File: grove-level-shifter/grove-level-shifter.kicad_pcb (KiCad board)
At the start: 2 copper layers, 21.6 x 45.7 mm, 14 parts, among them J1 In 1, J2 In 2, J3 Out 1, J4 Out 2, J5 Power, J6 In, J7 Out, J8 USB, J9 External Power, U1 TXB0108PW

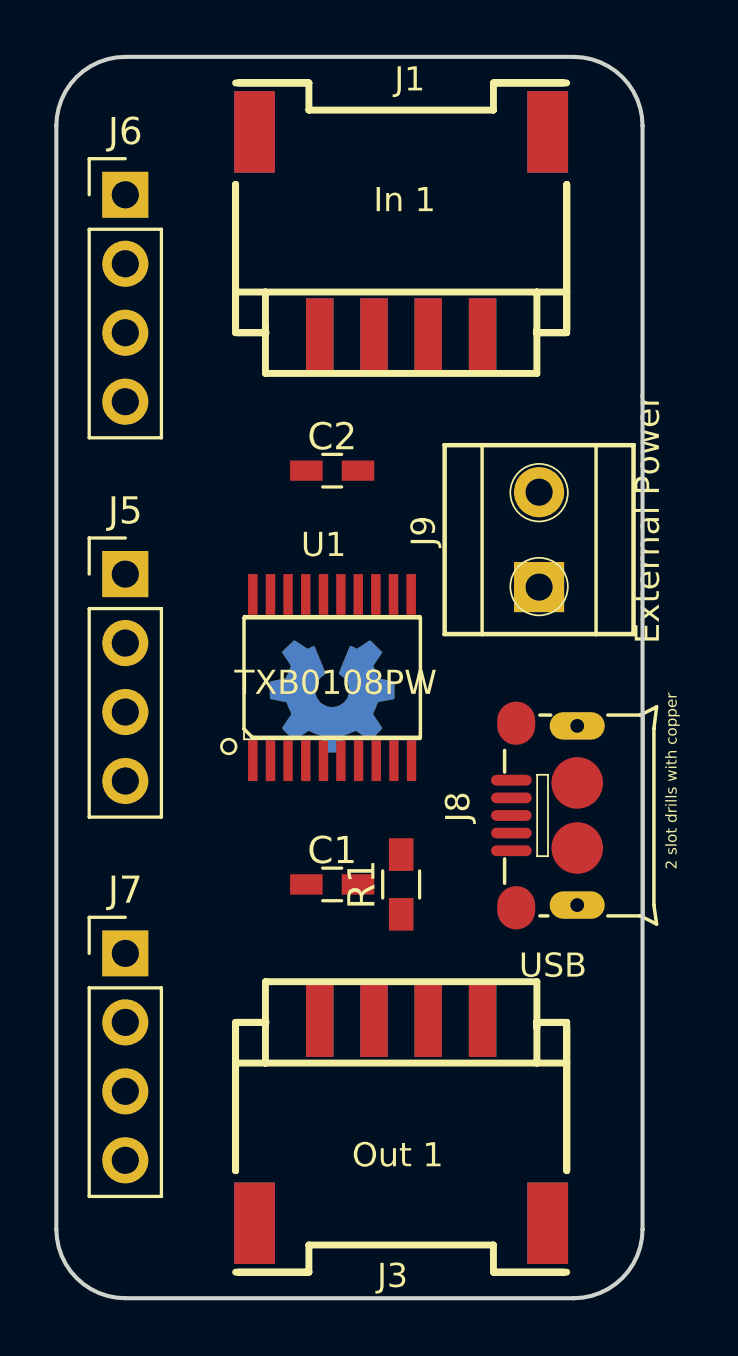
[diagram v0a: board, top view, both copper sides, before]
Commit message: Routed PCB
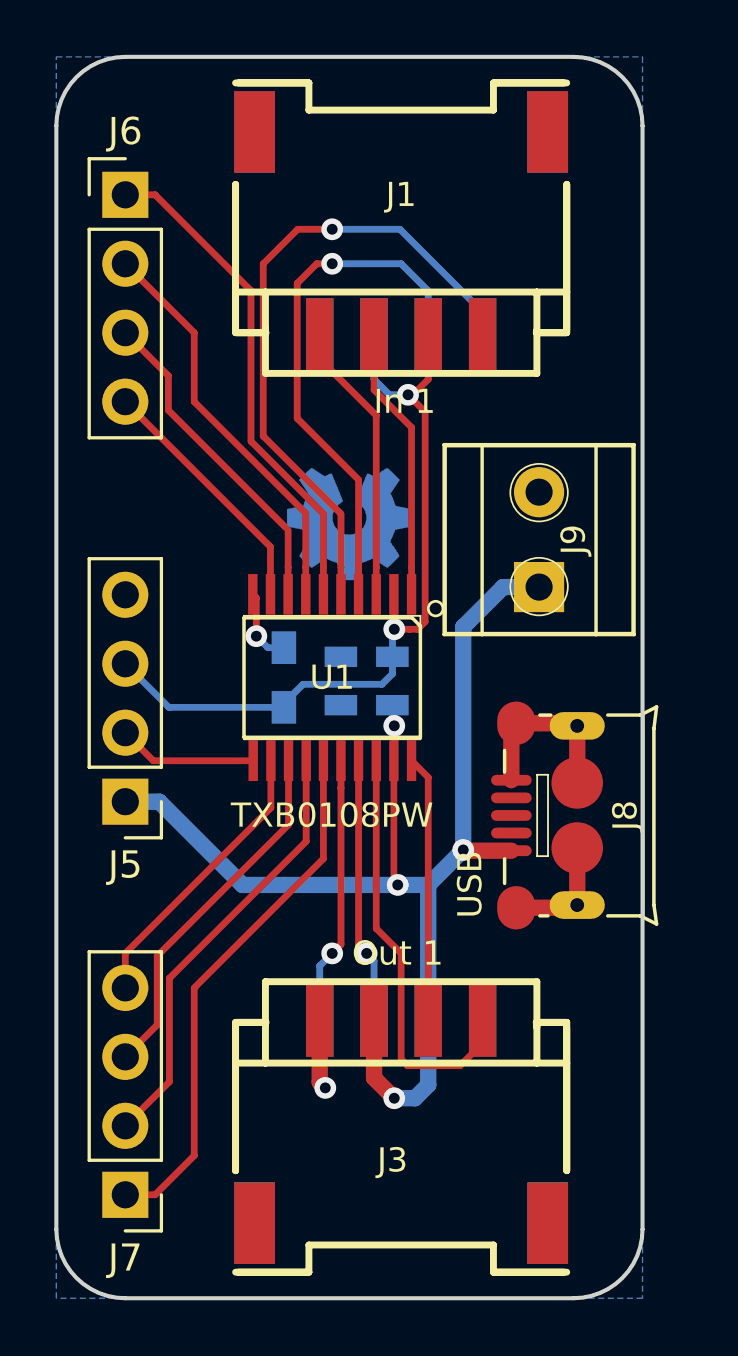
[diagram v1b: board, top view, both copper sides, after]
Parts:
- C1, C2, R1: moved to B.Cu
- moved J7 8.89 mm to (30.5, 67.3), turned to 180 degrees
- moved R1 8.76 mm to (36.3, 48.3)
- moved C2 8.73 mm to (39.4, 49.3), turned to 180 degrees
- moved C1 8.48 mm to (39.4, 47.5)
- moved J5 8.38 mm to (30.5, 52.8), turned to 180 degrees
- moved Z1 6.38 mm to (38.7, 41.9)
- turned U1 to 180 degrees
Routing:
- net +5V: track 0.00 -> 46.4 mm, vias 0 -> 4
- net +3V3: track 0.00 -> 29.6 mm, vias 0 -> 2
- net IN_2_DATA: track 0.00 -> 24.1 mm, vias 0 -> 1
- net Net-(J7-Pad1): track 0.00 -> 19.7 mm
- net IN_2_CLK: track 0.00 -> 19.6 mm, vias 0 -> 1
- net GND: track 0.00 -> 18.7 mm, vias 0 -> 1
- net Net-(J6-Pad1): track 0.00 -> 18.4 mm
- net Net-(J7-Pad2): track 0.00 -> 16.2 mm
- net OUT_1_DATA: track 0.00 -> 15.7 mm
- net Net-(J6-Pad2): track 0.00 -> 14.9 mm
- net Net-(J7-Pad3): track 0.00 -> 13.4 mm
- net Net-(J6-Pad3): track 0.00 -> 12.0 mm
- net Net-(J7-Pad4): track 0.00 -> 10.6 mm
- net IN_1_DATA: track 0.00 -> 10.4 mm
- net IN_1_CLK: track 0.00 -> 10.1 mm
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- added copper zone on B.Cu, net GND
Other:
- net class High Current added: clearance 0.3, trace_width 0.4, via_dia 0.8, via_drill 0.4
- board text added: "github.com/jimmo/microbit-boards/"
